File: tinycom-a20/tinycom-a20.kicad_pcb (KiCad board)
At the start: 4 copper layers, 41.7 x 40.9 mm, 37 parts, among them P1 CONN_02X10, P2 CONN_02X10, P3 CONN_01X01, P4 CONN_01X03, U1 ALLWINNERA10/TFBGA441, U2 H5TQG63BFR/FBGA96, Y1 Crystal_Small, Y2 Crystal_Small

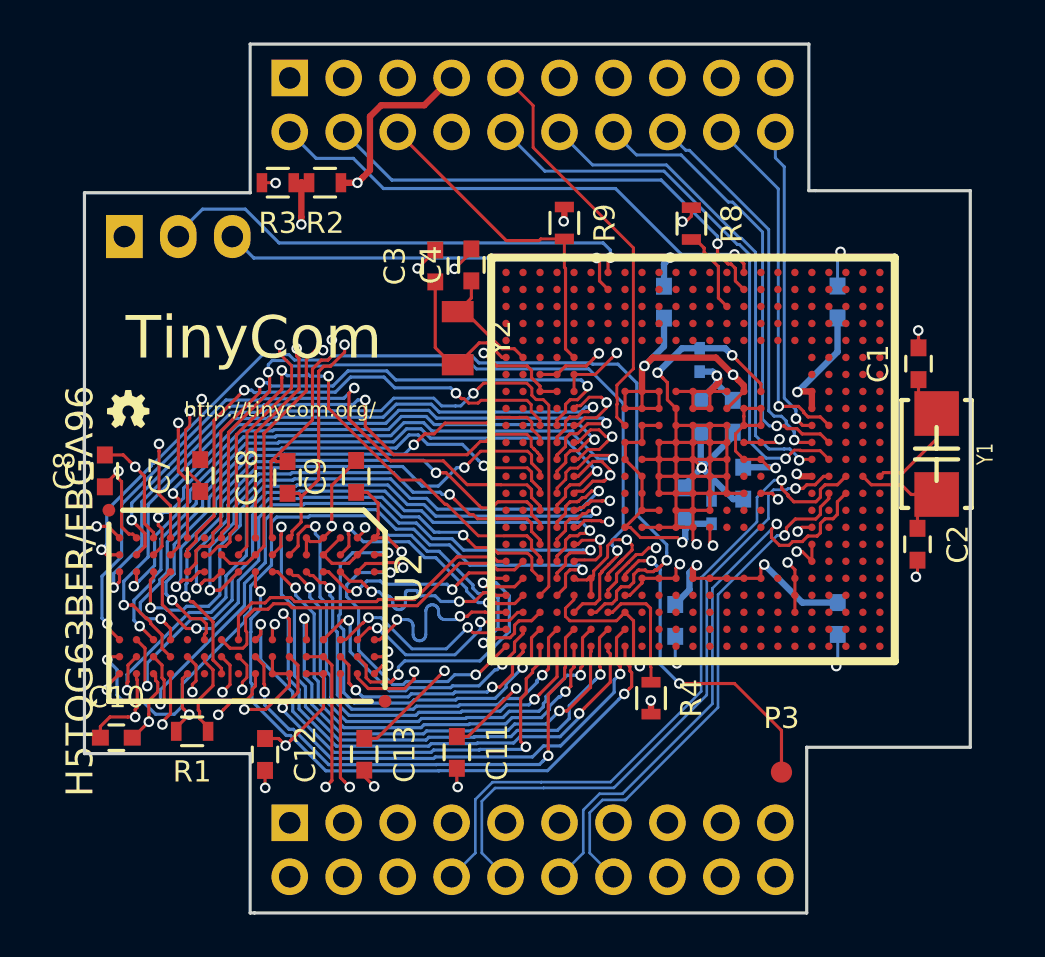
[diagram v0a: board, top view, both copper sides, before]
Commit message: pics
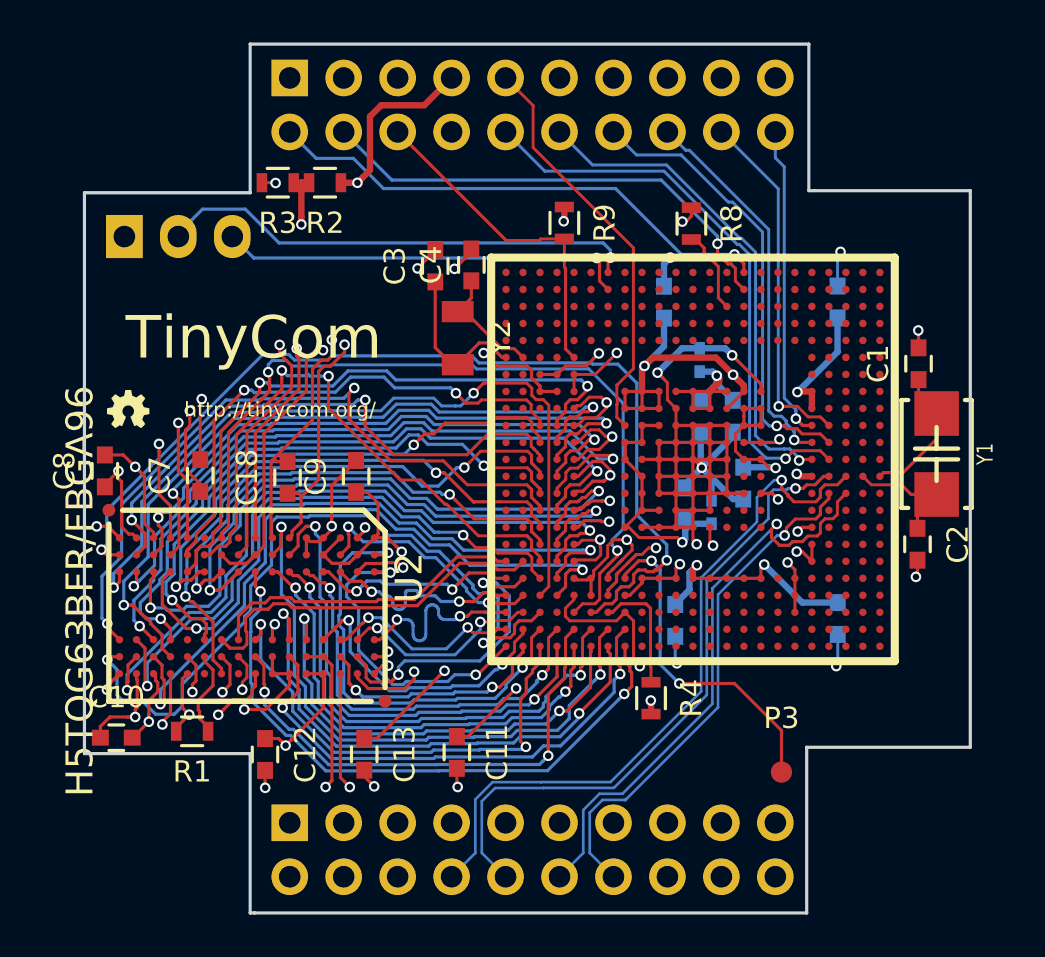
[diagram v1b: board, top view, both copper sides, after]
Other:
- rule pad_to_mask_clearance: 0.07 -> 0.065
